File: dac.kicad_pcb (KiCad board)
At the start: 2 copper layers, 52 x 31 mm, 21 parts, among them J1 RCJ-2121, J2 Conn_01x03_Male, SW1 SW_DIP_x01, U1 pcm5102a

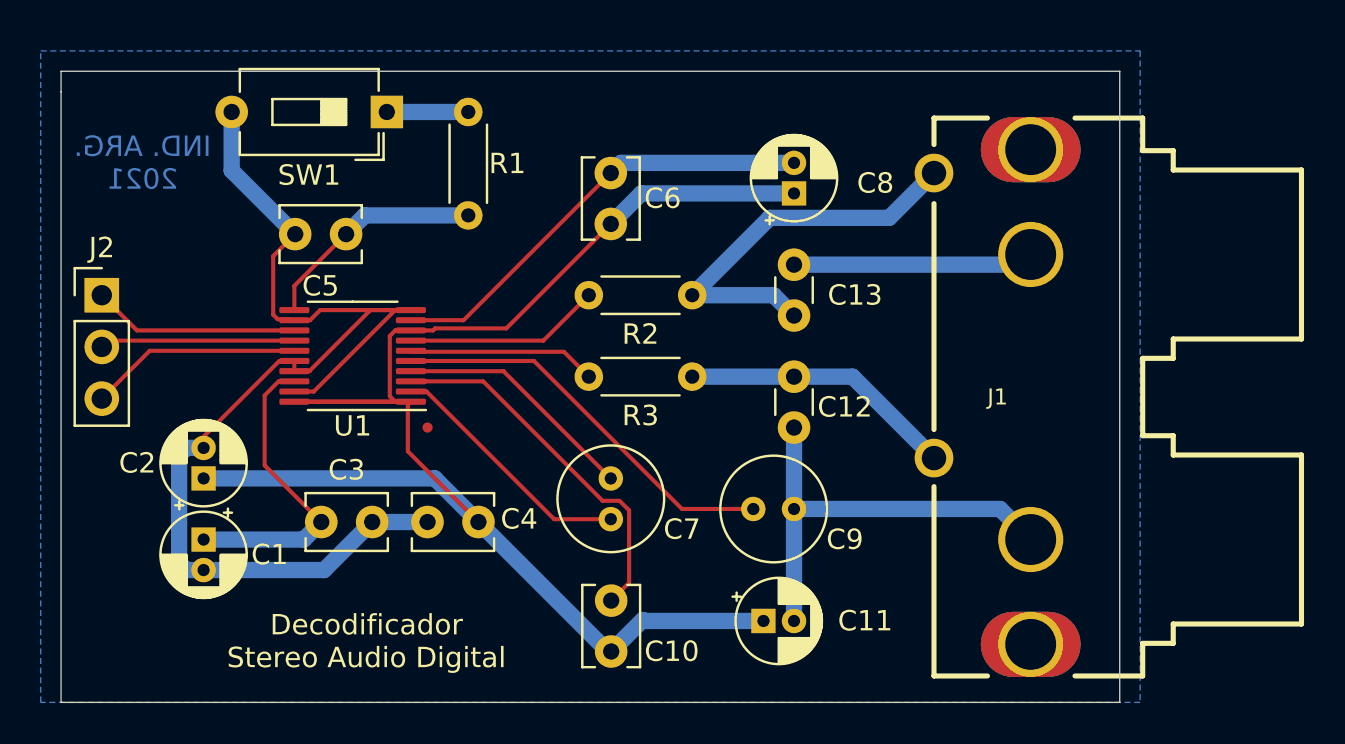
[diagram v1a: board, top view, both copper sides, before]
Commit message: pcb terminado
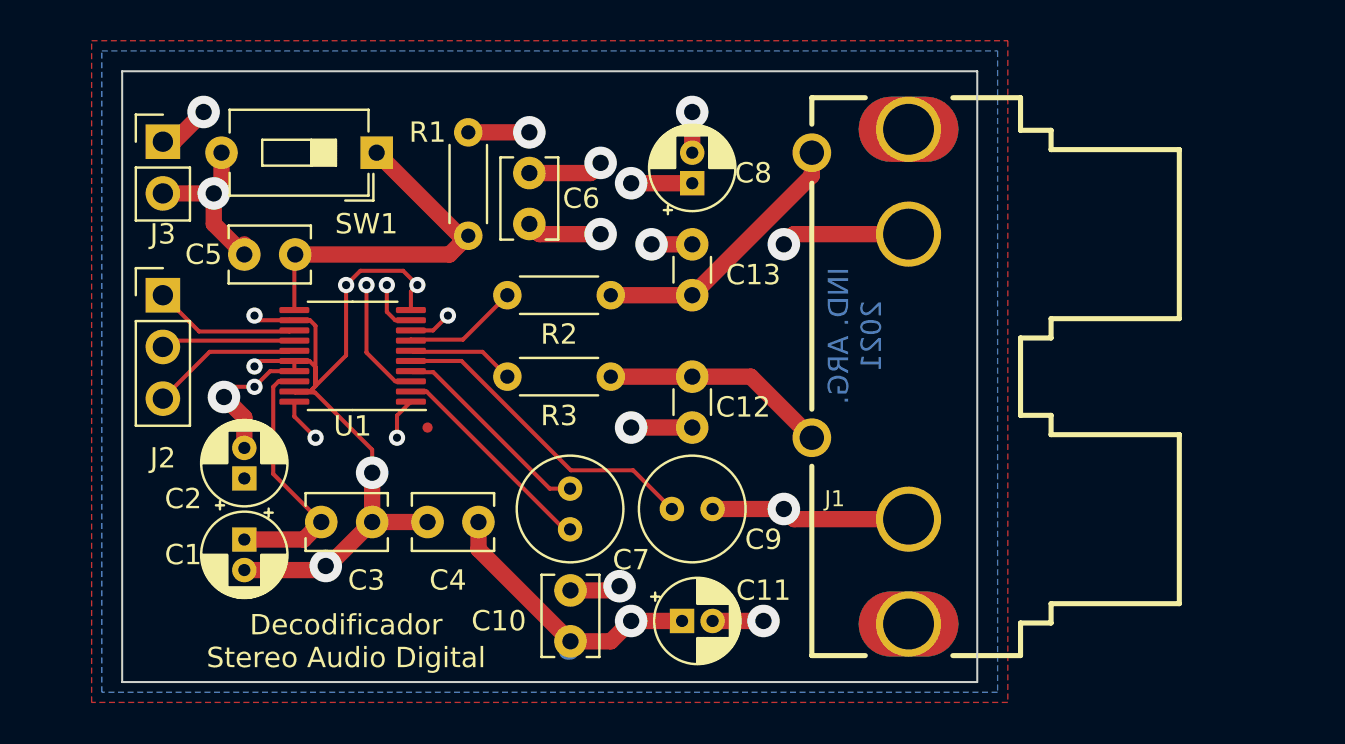
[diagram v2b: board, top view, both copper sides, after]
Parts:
- added J3: Conn_01x02_Male, Connector_PinHeader_2.54mm:PinHeader_1x02_P2.54mm_Vertical, F.Cu at (138.0, 83.5)
- moved J1 6.08 mm to (173.0, 95.0)
- moved C13 5.10 mm to (164.0, 91.0)
- moved C8 5.02 mm to (164.0, 85.5)
- moved C12 5.00 mm to (164.0, 95.0)
- moved C11 4.00 mm to (163.5, 107.0)
- moved C6 4.00 mm to (156.0, 85.0)
- moved C9 4.00 mm to (163.0, 101.5)
- moved R2 4.00 mm to (160.0, 91.0)
- moved R3 4.00 mm to (160.0, 95.0)
- moved J2 3.00 mm to (138.0, 91.0)
- moved C5 2.69 mm to (144.5, 89.0)
- moved C10 2.06 mm to (158.0, 105.5)
- moved C7 2.06 mm to (158.0, 100.5)
- moved SW1 2.06 mm to (148.5, 84.0)
- moved C1 2.00 mm to (142.0, 103.0)
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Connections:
- net Net-(R2-Pad2) renamed /OUTR
- net Net-(R3-Pad2) renamed /OUTL
- C1 pad 2: Earth -> GND
- C2 pad 2: Earth -> GND
- C3 pad 2: Earth -> GND
- C4 pad 1: Earth -> GND
- C5 pad 1: Net-(C5-Pad1) -> /FLT
- C5 pad 2: Earth -> GNDA
- R1 pad 1: Net-(R1-Pad1) -> +3.3VA
- R1 pad 2: Net-(C5-Pad1) -> /FLT
- SW1 pad 1: Net-(R1-Pad1) -> /FLT
- SW1 pad 2: Earth -> GNDA
- U1 pad 10: Earth -> GND
- U1 pad 11: Net-(C5-Pad1) -> /FLT
- U1 pad 12: Earth -> GND
- U1 pad 16: Earth -> GND
- U1 pad 17: Earth -> GND
- U1 pad 19: Earth -> GND
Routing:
- net Earth: track 60.9 -> 0.00 mm
- net GND: track 0.00 -> 49.4 mm, vias 0 -> 8
- net +3.3VA: track 76.6 -> 33.0 mm, vias 0 -> 8
- net GNDA: track 74.5 -> 49.6 mm, vias 0 -> 11
- net /FLT: track 0.00 -> 17.8 mm
- net Net-(C5-Pad1): track 11.2 -> 0.00 mm
- net Net-(C13-Pad1): track 19.8 -> 13.4 mm
- net Net-(R1-Pad1): track 4.00 -> 0.00 mm
- net /OUTR: track 9.66 -> 5.69 mm
- net /OUTL: track 9.26 -> 5.38 mm
- net Net-(C9-Pad1): track 19.8 -> 16.6 mm
- net Net-(J2-Pad2): track 9.59 -> 6.59 mm
- net Net-(J2-Pad3): track 10.4 -> 7.43 mm
- net Net-(J2-Pad1): track 10.2 -> 7.22 mm
- net Net-(C12-Pad1): track 13.5 -> 11.1 mm
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- added copper zone on F.Cu, net +3.3VA
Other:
- board size 52 x 31 mm -> 42 x 30 mm
- board text added: "Fabricante: Mayer Grilla: 1mm, 0,5mm Margen: 0,2mm Via: 1,6mm / 0,8mm, 0,8mm/0,40mm Pista: 0,2mm, 0,8mm Distancias al borde: 1mm Terminación superficial: HASL"
- board text removed: "Grilla: 1mm, 0,5mm Margen: 0,2mm Via: 1,6mm / 0,8mm Pista: 0,2mm, 0,8mm Distancias al borde: 1mm Terminacion: HASL"
